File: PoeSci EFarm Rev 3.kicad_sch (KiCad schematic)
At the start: 22 parts, among them J1 SIM_Card, J2 Conn_Coaxial, J3 Conn_01x08_Socket, J4 Conn_01x08_Socket, Q1 UMH3N, Q2 BSS138, Q3 BSS138, Q4 UMH3N, U1 UC200T

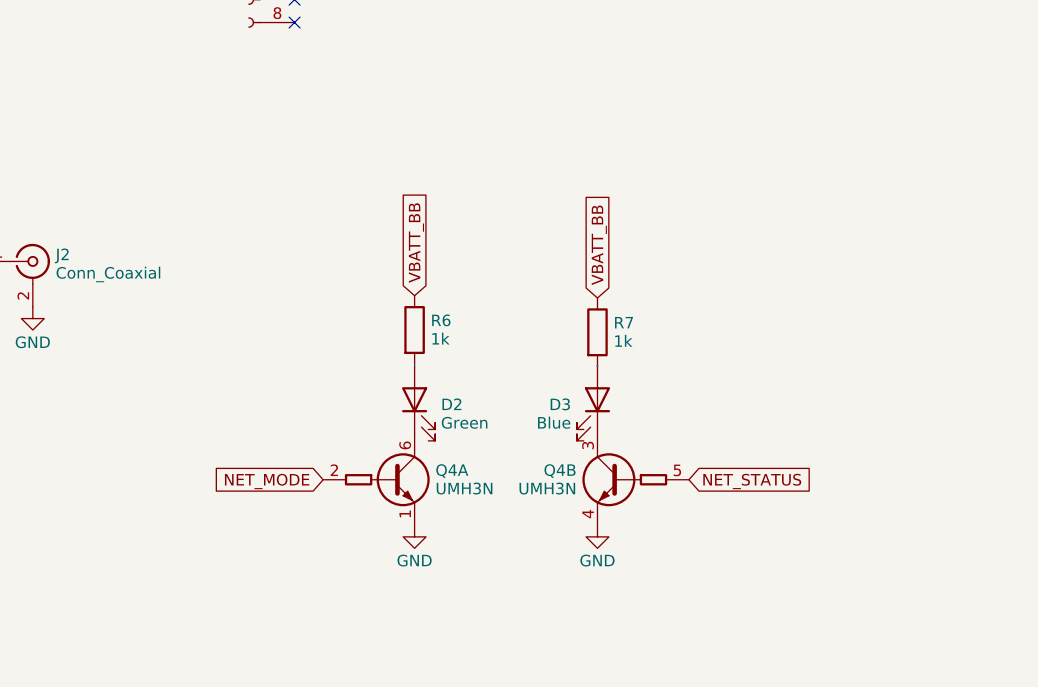
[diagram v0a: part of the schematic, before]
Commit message: Change position a bit
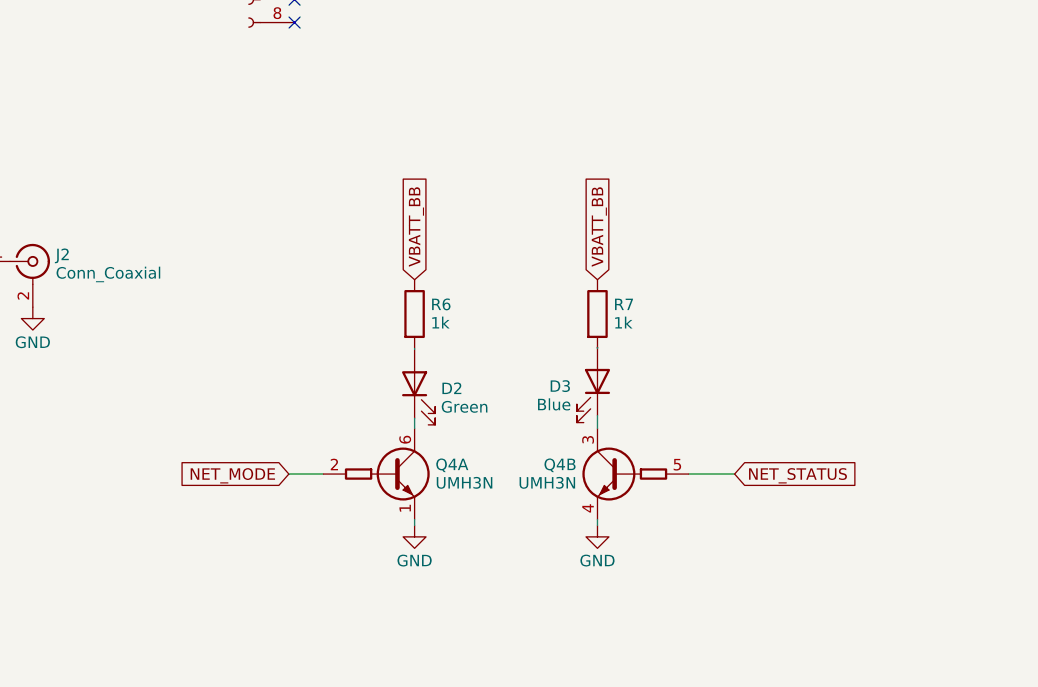
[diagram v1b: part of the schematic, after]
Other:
- moved on the sheet: D2, D3, Q4A, Q4B, R6, R7
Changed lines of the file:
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@@
 	(wire
 		(pts
+			(xy 257.81 165.1) (xy 257.81 165.735)
+		)
+		(stroke
+			(width 0)
+			(type default)
+		)
+	)
+	(wire
+		(pts
+			(xy 278.13 165.1) (xy 278.13 165.735)
+		)
+		(stroke
+			(width 0)
+			(type default)
+		)
+	)
+	(wire
+		(pts
 			(xy 389.255 57.15) (xy 389.255 62.23)
 		)
@@
 	(wire
 		(pts
-			(xy 278.13 148.082) (xy 278.13 147.955)
+			(xy 278.13 146.05) (xy 278.13 145.923)
+		)
+		(stroke
+			(width 0)
+			(type default)
+		)
+	)
+	(wire
+		(pts
+			(xy 243.84 160.02) (xy 247.65 160.02)
 		)
 		(stroke
@@
 	(wire
 		(pts
-			(xy 257.81 147.828) (xy 257.81 147.955)
+			(xy 257.81 146.05) (xy 257.81 146.177)
 		)
 		(stroke
@@
 	(wire
 		(pts
+			(xy 257.81 153.797) (xy 257.81 154.94)
+		)
+		(stroke
+			(width 0)
+			(type default)
+		)
+	)
+	(wire
+		(pts
 			(xy 200.152 121.158) (xy 206.502 121.158)
 		)
@@
 	(wire
 		(pts
+			(xy 293.37 160.02) (xy 288.29 160.02)
+		)
+		(stroke
+			(width 0)
+			(type default)
+		)
+	)
+	(wire
+		(pts
 			(xy 389.255 77.47) (xy 389.255 82.55)
 		)
@@
 		)
 	)
+	(wire
+		(pts
+			(xy 278.13 154.94) (xy 278.13 153.543)
+		)
+		(stroke
+			(width 0)
+			(type default)
+		)
+	)
 	(label "USIM_VDD"
 		(at 51.308 234.95 0)
@@
 	(global_label "NET_MODE"
 		(shape input)
-		(at 247.65 160.655 180)
+		(at 243.84 160.02 180)
 		(fields_autoplaced yes)
 		(effects
@@
 		)
 		(property "Intersheetrefs" "${INTERSHEET_REFS}"
-			(at 235.1286 160.655 0)
+			(at 231.3186 160.02 0)
 			(effects
 				(font
@@
 	(global_label "VBATT_BB"
 		(shape input)
-		(at 278.13 140.462 90)
+		(at 278.13 138.43 90)
 		(fields_autoplaced yes)
 		(effects
@@
 		)
 		(property "Intersheetrefs" "${INTERSHEET_REFS}"
-			(at 278.13 128.6662 90)
+			(at 278.13 126.6342 90)
 			(effects
 				(font
@@
 	(global_label "NET_STATUS"
 		(shape input)
-		(at 288.29 160.655 0)
+		(at 293.37 160.02 0)
 		(fields_autoplaced yes)
 		(effects
@@
 		)
 		(property "Intersheetrefs" "${INTERSHEET_REFS}"
-			(at 302.3838 160.655 0)
+			(at 307.4638 160.02 0)
 			(effects
 				(font
@@
 	(global_label "VBATT_BB"
 		(shape input)
-		(at 257.81 140.208 90)
+		(at 257.81 138.43 90)
 		(fields_autoplaced yes)
 		(effects
@@
 		)
 		(property "Intersheetrefs" "${INTERSHEET_REFS}"
-			(at 257.81 128.4122 90)
+			(at 257.81 126.6342 90)
 			(effects
 				(font
@@
 	(symbol
 		(lib_id "Device:LED")
-		(at 278.13 151.765 270)
+		(at 278.13 149.733 270)
 		(mirror x)
 		(unit 1)
@@
 		(fields_autoplaced yes)
 		(property "Reference" "D3"
-			(at 275.209 152.3285 90)
+			(at 275.209 150.2965 90)
 			(effects
 				(font
@@
 		)
 		(property "Value" "Blue"
-			(at 275.209 154.3765 90)
+			(at 275.209 152.3445 90)
 			(effects
 				(font
@@
 		)
 		(property "Footprint" "LED_SMD:LED_0603_1608Metric_Pad1.05x0.95mm_HandSolder"
-			(at 278.13 151.765 0)
+			(at 278.13 149.733 0)
 			(effects
 				(font
@@
 		)
 		(property "Datasheet" "~"
-			(at 278.13 151.765 0)
+			(at 278.13 149.733 0)
 			(effects
 				(font
@@
 		)
 		(property "Description" ""
-			(at 278.13 151.765 0)
+			(at 278.13 149.733 0)
 			(effects
 				(font
@@
 	(symbol
 		(lib_id "Device:R")
-		(at 257.81 144.018 0)
+		(at 257.81 142.24 0)
 		(unit 1)
 		(exclude_from_sim no)
@@
 		(fields_autoplaced yes)
 		(property "Reference" "R6"
-			(at 259.588 142.994 0)
+			(at 259.588 141.216 0)
 			(effects
 				(font
@@
 		)
 		(property "Value" "1k"
-			(at 259.588 145.042 0)
+			(at 259.588 143.264 0)
 			(effects
 				(font
@@
 		)
 		(property "Footprint" "Resistor_SMD:R_0603_1608Metric_Pad0.98x0.95mm_HandSolder"
-			(at 256.032 144.018 90)
+			(at 256.032 142.24 90)
 			(effects
 				(font
@@
 		)
 		(property "Datasheet" "~"
-			(at 257.81 144.018 0)
+			(at 257.81 142.24 0)
 			(effects
 				(font
@@
 		)
 		(property "Description" ""
-			(at 257.81 144.018 0)
+			(at 257.81 142.24 0)
 			(effects
 				(font
@@
 	(symbol
 		(lib_id "Device:LED")
-		(at 257.81 151.765 90)
+		(at 257.81 149.987 90)
 		(unit 1)
 		(exclude_from_sim no)
@@
 		(fields_autoplaced yes)
 		(property "Reference" "D2"
-			(at 260.731 152.3285 90)
+			(at 260.731 150.5505 90)
 			(effects
 				(font
@@
 		)
 		(property "Value" "Green"
-			(at 260.731 154.3765 90)
+			(at 260.731 152.5985 90)
 			(effects
 				(font
@@
 		)
 		(property "Footprint" "LED_SMD:LED_0603_1608Metric_Pad1.05x0.95mm_HandSolder"
-			(at 257.81 151.765 0)
+			(at 257.81 149.987 0)
 			(effects
 				(font
@@
 		)
 		(property "Datasheet" "~"
-			(at 257.81 151.765 0)
+			(at 257.81 149.987 0)
 			(effects
 				(font
@@
 		)
 		(property "Description" ""
-			(at 257.81 151.765 0)
+			(at 257.81 149.987 0)
 			(effects
 				(font
@@
 	(symbol
 		(lib_id "Device:R")
-		(at 278.13 144.272 0)
+		(at 278.13 142.24 0)
 		(unit 1)
 		(exclude_from_sim no)
@@
 		(fields_autoplaced yes)
 		(property "Reference" "R7"
-			(at 279.908 143.248 0)
+			(at 279.908 141.216 0)
 			(effects
 				(font
@@
 		)
 		(property "Value" "1k"
-			(at 279.908 145.296 0)
+			(at 279.908 143.264 0)
 			(effects
 				(font
@@
 		)
 		(property "Footprint" "Resistor_SMD:R_0603_1608Metric_Pad0.98x0.95mm_HandSolder"
-			(at 276.352 144.272 90)
+			(at 276.352 142.24 90)
 			(effects
 				(font
@@
 		)
 		(property "Datasheet" "~"
-			(at 278.13 144.272 0)
+			(at 278.13 142.24 0)
 			(effects
 				(font
@@
 		)
 		(property "Description" ""
-			(at 278.13 144.272 0)
+			(at 278.13 142.24 0)
 			(effects
 				(font
@@
 	(symbol
 		(lib_id "Transistor_BJT:UMH3N")
-		(at 252.73 160.655 0)
+		(at 252.73 160.02 0)
 		(unit 1)
 		(exclude_from_sim no)
@@
 		(fields_autoplaced yes)
 		(property "Reference" "Q4"
-			(at 260.1214 159.631 0)
+			(at 260.1214 158.996 0)
 			(effects
 				(font
@@
 		)
 		(property "Value" "UMH3N"
-			(at 260.1214 161.679 0)
+			(at 260.1214 161.044 0)
 			(effects
 				(font
@@
 		)
 		(property "Footprint" "Package_TO_SOT_SMD:SOT-363_SC-70-6"
-			(at 252.857 171.831 0)
+			(at 252.857 171.196 0)
 			(effects
 				(font
@@
 		)
 		(property "Datasheet" "http://rohmfs.rohm.com/en/products/databook/datasheet/discrete/transistor/digital/emh3t2r-e.pdf"
-			(at 256.54 160.655 0)
+			(at 256.54 160.02 0)
 			(effects
 				(font
@@
 		)
 		(property "Description" ""
-			(at 252.73 160.655 0)
+			(at 252.73 160.02 0)
 			(effects
 				(font
@@
 	(symbol
 		(lib_id "Transistor_BJT:UMH3N")
-		(at 283.21 160.655 0)
+		(at 283.21 160.02 0)
 		(mirror y)
 		(unit 2)
@@
 		(fields_autoplaced yes)
 		(property "Reference" "Q4"
-			(at 275.8186 159.631 0)
+			(at 275.8186 158.996 0)
 			(effects
 				(font
@@
 		)
 		(property "Value" "UMH3N"
-			(at 275.8186 161.679 0)
+			(at 275.8186 161.044 0)
 			(effects
 				(font
@@
 		)
 		(property "Footprint" "Package_TO_SOT_SMD:SOT-363_SC-70-6"
-			(at 283.083 171.831 0)
+			(at 283.083 171.196 0)
 			(effects
 				(font
@@
 		)
 		(property "Datasheet" "http://rohmfs.rohm.com/en/products/databook/datasheet/discrete/transistor/digital/emh3t2r-e.pdf"
-			(at 279.4 160.655 0)
+			(at 279.4 160.02 0)
 			(effects
 				(font
@@
 		)
 		(property "Description" ""
-			(at 283.21 160.655 0)
+			(at 283.21 160.02 0)
 			(effects
 				(font
